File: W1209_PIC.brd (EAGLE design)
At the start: 49 x 40 mm, 41 parts, among them IC1 MCP1825S-33, IC2 PIC18F14K50SS, K1 JJM1A-12V, Q1 BC817-40SMD, X1 MKDSN1,5/2-5,08, X3 NTC, X4 53047-05, X5 MKDSN1,5/2-5,08

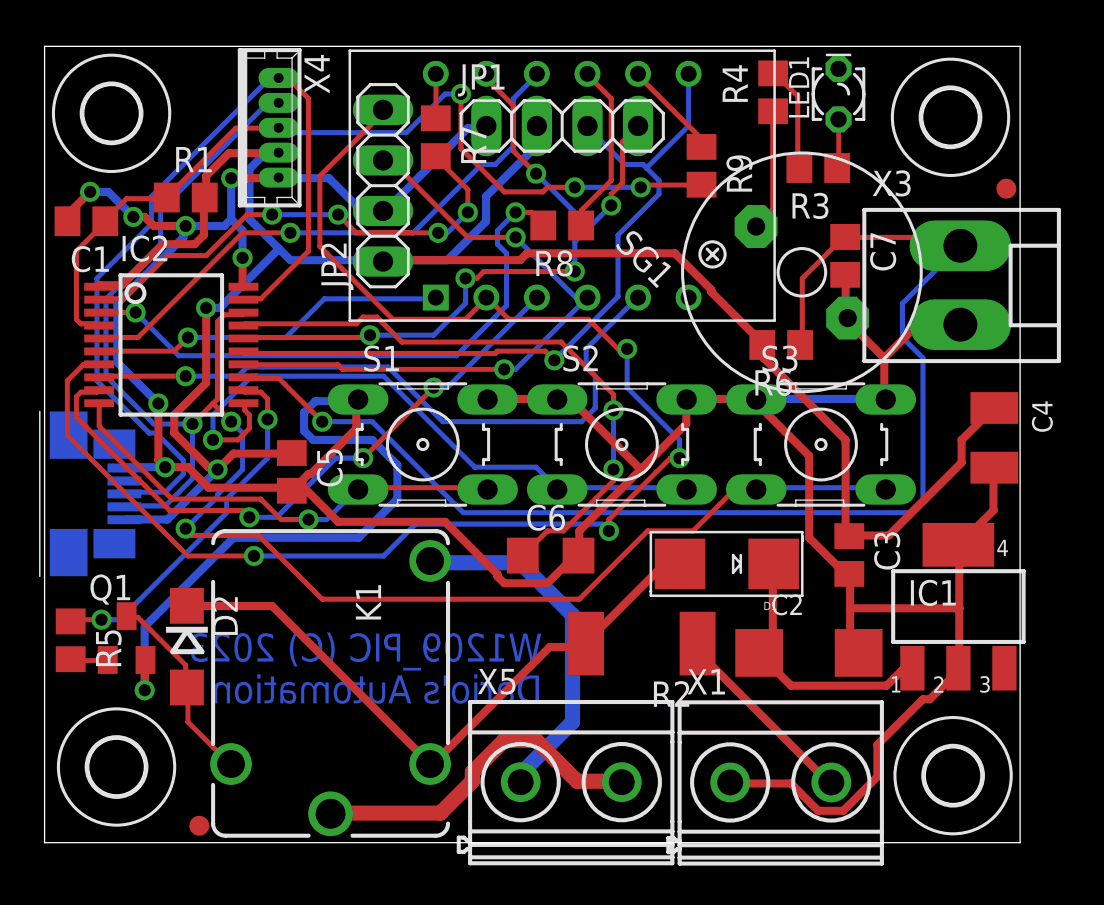
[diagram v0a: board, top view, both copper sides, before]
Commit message: Add files via upload
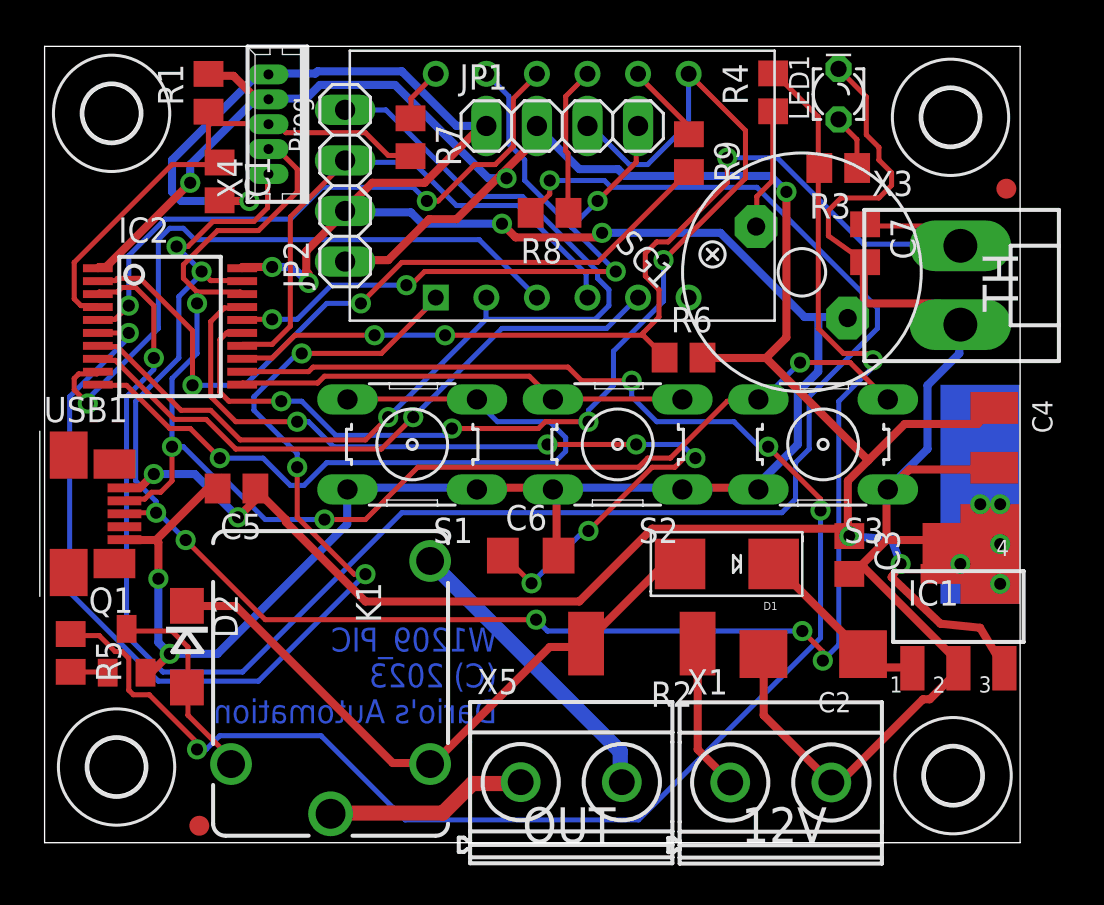
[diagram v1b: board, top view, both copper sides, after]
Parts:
- moved C1 6.98 mm to (8.79, 33.2), turned to 270 degrees
- moved R1 5.38 mm to (8.23, 37.7), turned to 90 degrees
- moved R6 4.95 mm to (32.1, 24.4), turned to 0 degrees
- moved C5 2.90 mm to (9.64, 17.8), turned to 180 degrees
- moved JP2 1.90 mm to (15.1, 33.0)
- moved R7 1.27 mm to (18.4, 35.4)
- moved C7 1.18 mm to (41.2, 30.1)
- moved C6 1.00 mm to (24.4, 14.4)
- moved R3 1.00 mm to (39.9, 33.9)
- moved USB1 1.00 mm to (1.21, 16.5), flipped to the top, turned to 0 degrees
- moved IC2 0.93 mm to (6.30, 25.9)
- moved R8 0.90 mm to (25.4, 31.6)
- moved R9 0.90 mm to (32.4, 34.6)
- moved Q1 0.63 mm to (4.12, 9.64)
- moved R5 0.63 mm to (1.31, 9.53)
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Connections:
- net GND: now also X1.2; no longer X1.1
- net K1: now also C1.1, IC2.4, R1.1, X4.3; no longer IC2.2
- net K3: now also IC2.2; no longer C1.1, IC2.4, R1.1, X4.3
- net N$3: now also X5.1; no longer X5.2
- net N$4: now also X5.2; no longer X5.1
- net N$6: now also X1.1; no longer X1.2
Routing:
- net RELE: track 18.1 -> 86.4 mm, vias 2 -> 4
- net K2: track 29.4 -> 90.9 mm
- net D+: track 48.5 -> 96.8 mm, vias 0 -> 8
- net SEG_E: track 18.0 -> 57.6 mm, vias 1 -> 4
- net +5V: track 105.2 -> 143.7 mm, vias 2 -> 7
- net SEG_D: track 73.9 -> 49.5 mm, vias 4 -> 1
- net SEG_B: track 37.5 -> 54.8 mm, vias 1 -> 4
- net SW3: track 84.0 -> 68.5 mm, vias 3 -> 4
- net SW1: track 23.3 -> 38.8 mm
- net N$15: track 30.8 -> 44.2 mm, vias 2 -> 6
- net AN0: track 64.0 -> 52.6 mm, vias 1 -> 3
- net SW2: track 31.8 -> 22.8 mm, vias 1 -> 0
- net N$3: track 17.3 -> 10.2 mm
- net GND: track 196.9 -> 203.7 mm, vias 8 -> 7
- net K3: track 43.4 -> 38.0 mm, vias 3 -> 2
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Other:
- board text added: "12V"
- board text added: "OUT"
- board text added: "Prog"
- board text added: "TH"
